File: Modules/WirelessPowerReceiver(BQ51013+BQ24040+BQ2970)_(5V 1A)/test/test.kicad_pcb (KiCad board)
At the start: 2 copper layers, 32.4 x 17.1 mm, 12 parts, among them J1 Conn_01x02, J7 Conn_01x14

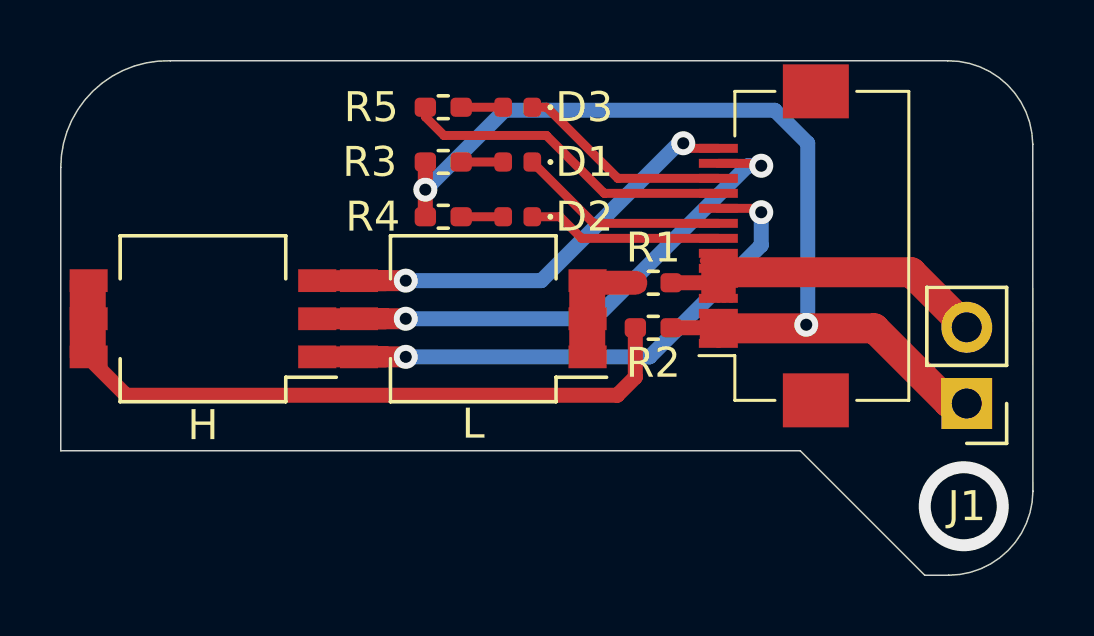
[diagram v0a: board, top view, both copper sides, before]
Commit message: Sort Out
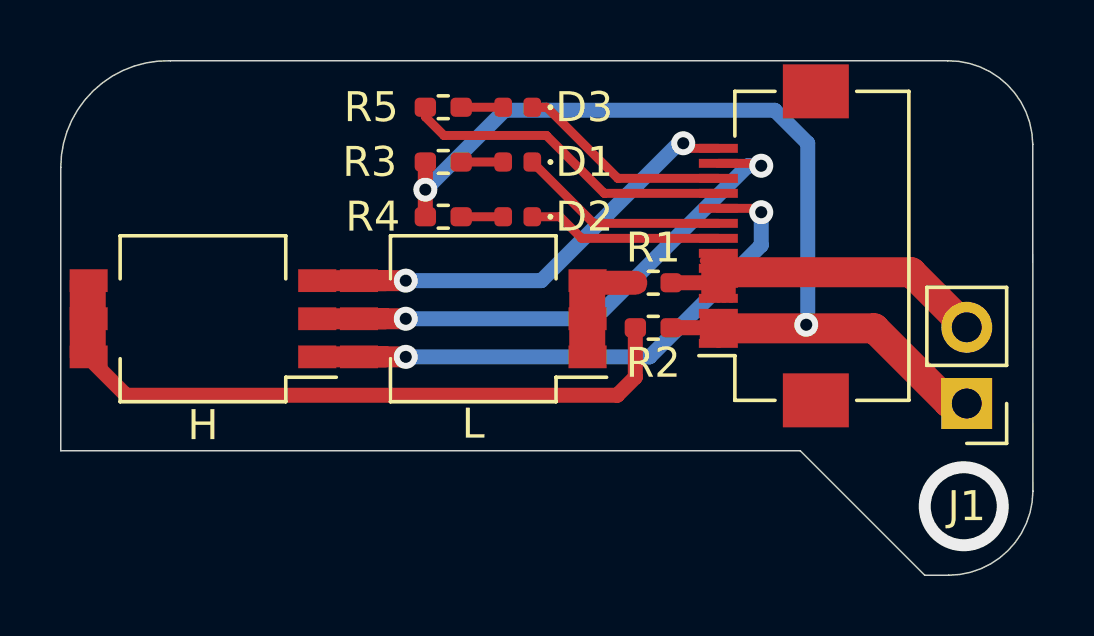
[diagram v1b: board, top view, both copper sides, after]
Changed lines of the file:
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@@
     )
     (pad_to_mask_clearance 0)
-    (aux_axis_origin 121.61 135.79)
-    (grid_origin 121.61 135.79)
+    (aux_axis_origin 154.07 125.22)
+    (grid_origin 154.07 125.22)
     (pcbplotparams
       (layerselection 0x00010fc_ffffffff)
@@
       (effects (font (size 1 1) (thickness 0.15)))
     )
-    (fp_line (start 5.15 4.5) (end 5.15 2.76) (layer "F.SilkS") (width 0.1))
-    (fp_line (start -5.15 -1.3) (end -5.15 0.04) (layer "F.SilkS") (width 0.1))
-    (fp_line (start 5.15 -1.3) (end 5.15 0.04) (layer "F.SilkS") (width 0.1))
-    (fp_line (start -5.15 2.76) (end -5.15 4.5) (layer "F.SilkS") (width 0.1))
-    (fp_line (start 3.66 -1.3) (end 5.15 -1.3) (layer "F.SilkS") (width 0.1))
-    (fp_line (start -3.66 -1.3) (end -3.66 -2.5) (layer "F.SilkS") (width 0.1))
-    (fp_line (start -3.66 -1.3) (end -5.15 -1.3) (layer "F.SilkS") (width 0.1))
-    (fp_line (start -5.15 4.5) (end 5.15 4.5) (layer "F.SilkS") (width 0.1))
+    (fp_line (start 5.15 -1.3) (end 5.15 0.04) (layer "F.SilkS") (width 0.12))
+    (fp_line (start 5.15 4.5) (end 5.15 2.76) (layer "F.SilkS") (width 0.12))
+    (fp_line (start -5.15 2.76) (end -5.15 4.5) (layer "F.SilkS") (width 0.12))
+    (fp_line (start 3.66 -1.3) (end 5.15 -1.3) (layer "F.SilkS") (width 0.12))
+    (fp_line (start -3.66 -1.3) (end -3.66 -2.5) (layer "F.SilkS") (width 0.12))
+    (fp_line (start -3.66 -1.3) (end -5.15 -1.3) (layer "F.SilkS") (width 0.12))
+    (fp_line (start -5.15 -1.3) (end -5.15 0.04) (layer "F.SilkS") (width 0.12))
+    (fp_line (start -5.15 4.5) (end 5.15 4.5) (layer "F.SilkS") (width 0.12))
+    (fp_line (start 6.55 -3) (end -6.55 -3) (layer "F.CrtYd") (width 0.05))
     (fp_line (start -6.55 4.9) (end 6.55 4.9) (layer "F.CrtYd") (width 0.05))
-    (fp_line (start 6.55 -3) (end -6.55 -3) (layer "F.CrtYd") (width 0.05))
+    (fp_line (start 6.55 4.9) (end 6.55 -3) (layer "F.CrtYd") (width 0.05))
     (fp_line (start -6.55 -3) (end -6.55 4.9) (layer "F.CrtYd") (width 0.05))
-    (fp_line (start 6.55 4.9) (end 6.55 -3) (layer "F.CrtYd") (width 0.05))
+    (fp_line (start 4.45 3.4) (end 4.45 3.7) (layer "F.Fab") (width 0.1))
     (fp_line (start 4.95 3.7) (end 4.95 4.4) (layer "F.Fab") (width 0.1))
+    (fp_line (start 5.05 -1.2) (end 5.05 3.4) (layer "F.Fab") (width 0.1))
+    (fp_line (start -4.95 3.7) (end -4.95 4.4) (layer "F.Fab") (width 0.1))
+    (fp_line (start -5.05 -1.2) (end -5.05 3.4) (layer "F.Fab") (width 0.1))
+    (fp_line (start 0 -1.2) (end 5.05 -1.2) (layer "F.Fab") (width 0.1))
+    (fp_line (start 4.95 4.4) (end 0 4.4) (layer "F.Fab") (width 0.1))
+    (fp_line (start -3.25 -0.492893) (end -2.75 -1.2) (layer "F.Fab") (width 0.1))
     (fp_line (start -3.75 -1.2) (end -3.25 -0.492893) (layer "F.Fab") (width 0.1))
-    (fp_line (start -4.95 3.7) (end -4.95 4.4) (layer "F.Fab") (width 0.1))
     (fp_line (start 5.05 3.4) (end 4.45 3.4) (layer "F.Fab") (width 0.1))
+    (fp_line (start 4.45 3.7) (end 4.95 3.7) (layer "F.Fab") (width 0.1))
+    (fp_line (start -5.05 3.4) (end -4.45 3.4) (layer "F.Fab") (width 0.1))
+    (fp_line (start -4.95 4.4) (end 0 4.4) (layer "F.Fab") (width 0.1))
+    (fp_line (start -4.45 3.7) (end -4.95 3.7) (layer "F.Fab") (width 0.1))
+    (fp_line (start -4.45 3.4) (end -4.45 3.7) (layer "F.Fab") (width 0.1))
     (fp_line (start 0 -1.2) (end -5.05 -1.2) (layer "F.Fab") (width 0.1))
-    (fp_line (start 0 -1.2) (end 5.05 -1.2) (layer "F.Fab") (width 0.1))
-    (fp_line (start 5.05 -1.2) (end 5.05 3.4) (layer "F.Fab") (width 0.1))
-    (fp_line (start 4.45 3.4) (end 4.45 3.7) (layer "F.Fab") (width 0.1))
-    (fp_line (start 4.95 4.4) (end 0 4.4) (layer "F.Fab") (width 0.1))
-    (fp_line (start -5.05 3.4) (end -4.45 3.4) (layer "F.Fab") (width 0.1))
-    (fp_line (start 4.45 3.7) (end 4.95 3.7) (layer "F.Fab") (width 0.1))
-    (fp_line (start -4.45 3.7) (end -4.95 3.7) (layer "F.Fab") (width 0.1))
-    (fp_line (start -4.95 4.4) (end 0 4.4) (layer "F.Fab") (width 0.1))
-    (fp_line (start -3.25 -0.492893) (end -2.75 -1.2) (layer "F.Fab") (width 0.1))
-    (fp_line (start -4.45 3.4) (end -4.45 3.7) (layer "F.Fab") (width 0.1))
-    (fp_line (start -5.05 -1.2) (end -5.05 3.4) (layer "F.Fab") (width 0.1))
-    (pad "1" smd rect locked (at -3.25 -1.85 90) (size 0.3 1.3) (layers "F.Cu" "F.Paste" "F.Mask")
+    (pad "" smd rect (at 5.15 1.4 90) (size 1.8 2.2) (layers "F.Cu" "F.Paste" "F.Mask"))
+    (pad "" smd rect (at -5.15 1.4 90) (size 1.8 2.2) (layers "F.Cu" "F.Paste" "F.Mask"))
+    (pad "1" smd rect (at -3.25 -1.85 90) (size 0.3 1.3) (layers "F.Cu" "F.Paste" "F.Mask")
       (net 5 "BAT+") (pinfunction "Pin_1") (pintype "passive"))
-    (pad "2" smd rect locked (at -2.75 -1.85 90) (size 0.3 1.3) (layers "F.Cu" "F.Paste" "F.Mask")
+    (pad "2" smd rect (at -2.75 -1.85 90) (size 0.3 1.3) (layers "F.Cu" "F.Paste" "F.Mask")
       (net 5 "BAT+") (pinfunction "Pin_2") (pintype "passive"))
-    (pad "3" smd rect locked (at -2.25 -1.85 90) (size 0.3 1.3) (layers "F.Cu" "F.Paste" "F.Mask")
+    (pad "3" smd rect (at -2.25 -1.85 90) (size 0.3 1.3) (layers "F.Cu" "F.Paste" "F.Mask")
       (net 5 "BAT+") (pinfunction "Pin_3") (pintype "passive"))
-    (pad "4" smd rect locked (at -1.75 -1.85 90) (size 0.3 1.3) (layers "F.Cu" "F.Paste" "F.Mask")
+    (pad "4" smd rect (at -1.75 -1.85 90) (size 0.3 1.3) (layers "F.Cu" "F.Paste" "F.Mask")
       (net 4 "GND") (pinfunction "Pin_4") (pintype "passive"))
-    (pad "5" smd rect locked (at -1.25 -1.85 90) (size 0.3 1.3) (layers "F.Cu" "F.Paste" "F.Mask")
+    (pad "5" smd rect (at -1.25 -1.85 90) (size 0.3 1.3) (layers "F.Cu" "F.Paste" "F.Mask")
       (net 4 "GND") (pinfunction "Pin_5") (pintype "passive"))
-    (pad "6" smd rect locked (at -0.75 -1.85 90) (size 0.3 1.3) (layers "F.Cu" "F.Paste" "F.Mask")
+    (pad "6" smd rect (at -0.75 -1.85 90) (size 0.3 1.3) (layers "F.Cu" "F.Paste" "F.Mask")
       (net 4 "GND") (pinfunction "Pin_6") (pintype "passive"))
-    (pad "7" smd rect locked (at -0.25 -1.85 90) (size 0.3 1.3) (layers "F.Cu" "F.Paste" "F.Mask")
+    (pad "7" smd rect (at -0.25 -1.85 90) (size 0.3 1.3) (layers "F.Cu" "F.Paste" "F.Mask")
       (net 4 "GND") (pinfunction "Pin_7") (pintype "passive"))
-    (pad "8" smd rect locked (at 0.25 -1.85 90) (size 0.3 1.3) (layers "F.Cu" "F.Paste" "F.Mask")
+    (pad "8" smd rect (at 0.25 -1.85 90) (size 0.3 1.3) (layers "F.Cu" "F.Paste" "F.Mask")
       (net 14 "BAT_CHG") (pinfunction "Pin_8") (pintype "passive"))
-    (pad "9" smd rect locked (at 0.75 -1.85 90) (size 0.3 1.3) (layers "F.Cu" "F.Paste" "F.Mask")
+    (pad "9" smd rect (at 0.75 -1.85 90) (size 0.3 1.3) (layers "F.Cu" "F.Paste" "F.Mask")
       (net 13 "BAT_PG") (pinfunction "Pin_9") (pintype "passive"))
-    (pad "10" smd rect locked (at 1.25 -1.85 90) (size 0.3 1.3) (layers "F.Cu" "F.Paste" "F.Mask")
+    (pad "10" smd rect (at 1.25 -1.85 90) (size 0.3 1.3) (layers "F.Cu" "F.Paste" "F.Mask")
       (net 8 "BAT_ISET") (pinfunction "Pin_10") (pintype "passive"))
-    (pad "11" smd rect locked (at 1.75 -1.85 90) (size 0.3 1.3) (layers "F.Cu" "F.Paste" "F.Mask")
+    (pad "11" smd rect (at 1.75 -1.85 90) (size 0.3 1.3) (layers "F.Cu" "F.Paste" "F.Mask")
       (net 9 "REG_power") (pinfunction "Pin_11") (pintype "passive"))
-    (pad "12" smd rect locked (at 2.25 -1.85 90) (size 0.3 1.3) (layers "F.Cu" "F.Paste" "F.Mask")
+    (pad "12" smd rect (at 2.25 -1.85 90) (size 0.3 1.3) (layers "F.Cu" "F.Paste" "F.Mask")
       (net 12 "REG_CHG") (pinfunction "Pin_12") (pintype "passive"))
-    (pad "13" smd rect locked (at 2.75 -1.85 90) (size 0.3 1.3) (layers "F.Cu" "F.Paste" "F.Mask")
+    (pad "13" smd rect (at 2.75 -1.85 90) (size 0.3 1.3) (layers "F.Cu" "F.Paste" "F.Mask")
       (net 11 "REG_EN1") (pinfunction "Pin_13") (pintype "passive"))
-    (pad "14" smd rect locked (at 3.25 -1.85 90) (size 0.3 1.3) (layers "F.Cu" "F.Paste" "F.Mask")
+    (pad "14" smd rect (at 3.25 -1.85 90) (size 0.3 1.3) (layers "F.Cu" "F.Paste" "F.Mask")
       (net 10 "REG_EN2") (pinfunction "Pin_14") (pintype "passive"))
-    (pad "MP" smd rect locked (at 5.15 1.4 90) (size 1.8 2.2) (layers "F.Cu" "F.Paste" "F.Mask"))
-    (pad "MP" smd rect locked (at -5.15 1.4 90) (size 1.8 2.2) (layers "F.Cu" "F.Paste" "F.Mask"))
-    (model "${KISYS3DMOD}/Connector_FFC-FPC.3dshapes/Hirose_FH12-14S-0.5SH_1x14-1MP_P0.50mm_Horizontal.wrl"
+    (model "${KICAD6_3DMODEL_DIR}/Connector_FFC-FPC.3dshapes/Hirose_FH12-14S-0.5SH_1x14-1MP_P0.50mm_Horizontal.wrl"
       (offset (xyz 0 0 0))
       (scale (xyz 1 1 1))
@@
   (gr_line (start 188.71 112.570214) (end 188.715327 124.14) (layer "Edge.Cuts") (width 0.05))
   (gr_arc (start 156.31 113.34) (mid 157.38808 110.79704) (end 159.96 109.79) (layer "Edge.Cuts") (width 0.05))
-  (gr_arc (start 188.715327 124.14) (mid 187.887752 126.116182) (end 185.91 126.94) (layer "Edge.Cuts") (width 0.05))
+  (gr_arc (start 188.715327 124.14) (mid 187.887752 126.116183) (end 185.91 126.94) (layer "Edge.Cuts") (width 0.05))
   (gr_line (start 159.96 109.79) (end 185.879786 109.79) (layer "Edge.Cuts") (width 0.05))
   (gr_line (start 185.91 126.94) (end 185.11 126.94) (layer "Edge.Cuts") (width 0.05))
-  (gr_arc (start 185.879786 109.79) (mid 187.869341 110.595327) (end 188.71 112.570214) (layer "Edge.Cuts") (width 0.05))
+  (gr_arc (start 185.879786 109.79) (mid 187.869341 110.595328) (end 188.71 112.570214) (layer "Edge.Cuts") (width 0.05))
   (gr_line (start 156.31 122.79) (end 180.96 122.79) (layer "Edge.Cuts") (width 0.05))
   (gr_line (start 156.31 122.79) (end 156.31 113.34) (layer "Edge.Cuts") (width 0.05))
   (gr_line (start 180.96 122.79) (end 185.11 126.94) (layer "Edge.Cuts") (width 0.05))
-  (target plus (at 121.61 135.79) (size 5) (width 0.05) (layer "Edge.Cuts"))
+  (target plus (at 154.07 125.22) (size 5) (width 0.05) (layer "Edge.Cuts"))
   (via (at 186.41 124.64) (size 3) (drill 2.2) (layers "F.Cu" "B.Cu") (free) (net 0))
   (segment (start 169.6575 113.165) (end 171.0575 113.165) (width 0.3) (layer "F.Cu") (net 1))
